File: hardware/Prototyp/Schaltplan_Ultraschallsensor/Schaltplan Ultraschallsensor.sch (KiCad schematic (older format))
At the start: 21 parts, among them IC1 A5950, P1 CON-SENSOR2, P2 CONN_01X05, P3 CONN_01X01, P4 CONN_01X02, U1 XMC1XXX48, X1 CRYSTAL_3225

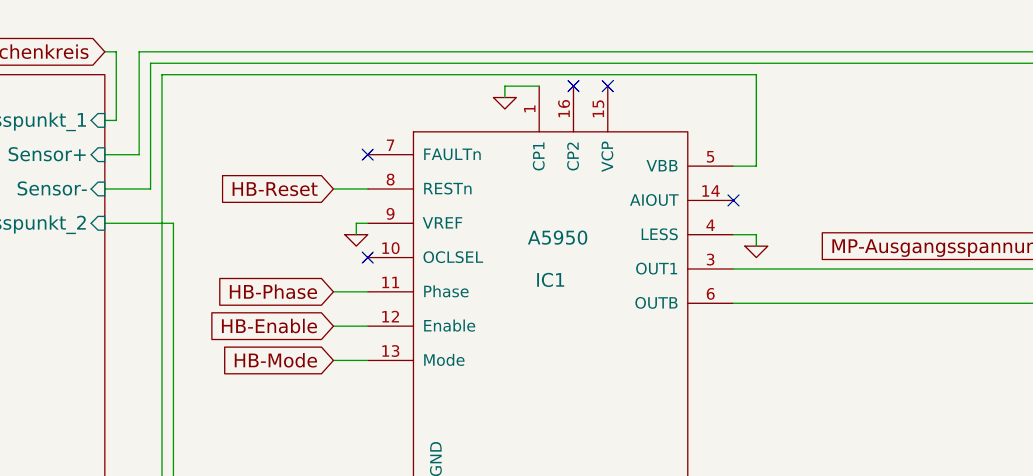
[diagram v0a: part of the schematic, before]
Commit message: Layout
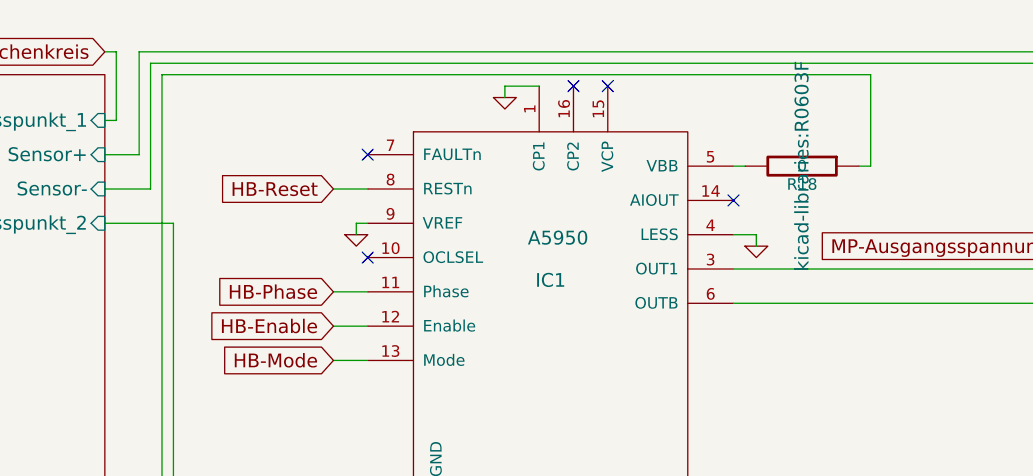
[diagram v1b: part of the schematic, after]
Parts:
- added R18: 0, kicad-libraries:R0603F, symbol R
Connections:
- net MP+Ua: now also R18.1; no longer IC1.5 (VBB)
- new net: IC1.5 (VBB), R18.2
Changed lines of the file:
@@
 Connection ~ 7150 1900
 Wire Wire Line
-	5250 1300 5150 1300
-Wire Wire Line
-	5250 900  5250 1300
-Wire Wire Line
-	2650 900  5250 900
+	2650 900  5750 900
 Wire Wire Line
 	2650 900  2650 3300
@@
 Wire Wire Line
 	5400 4050 5400 4100
+$Comp
+L R R18
+U 1 1 5A795B29
+P 5450 1300
+F 0 "R18" V 5530 1300 50  0000 C CNN
+F 1 "0" V 5450 1300 50  0000 C CNN
+F 2 "kicad-libraries:R0603F" H 5450 1300 60  0000 C CNN
+F 3 "" H 5450 1300 60  0000 C CNN
+	1    5450 1300
+	0    1    1    0
+$EndComp
+Wire Wire Line
+	5150 1300 5200 1300
+Wire Wire Line
+	5750 900  5750 1300
+Wire Wire Line
+	5750 1300 5700 1300
 $EndSCHEMATC
